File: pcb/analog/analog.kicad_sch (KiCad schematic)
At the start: 65 parts, among them J1 USB_C_Receptacle_USB2.0, SW1 SW_Push, SW2 SW_Push, U1 SRV05-4, U2 XC6206P332MR, U3 DRV5056A3xDBZxQ1, U4 DRV5056A3xDBZxQ1, U5 DRV5056A3xDBZxQ1, U6 74AHCT1G125, U7 74AHCT1G125, U8 RP2040, U9 W25Q128JVS, Y1 12MHz

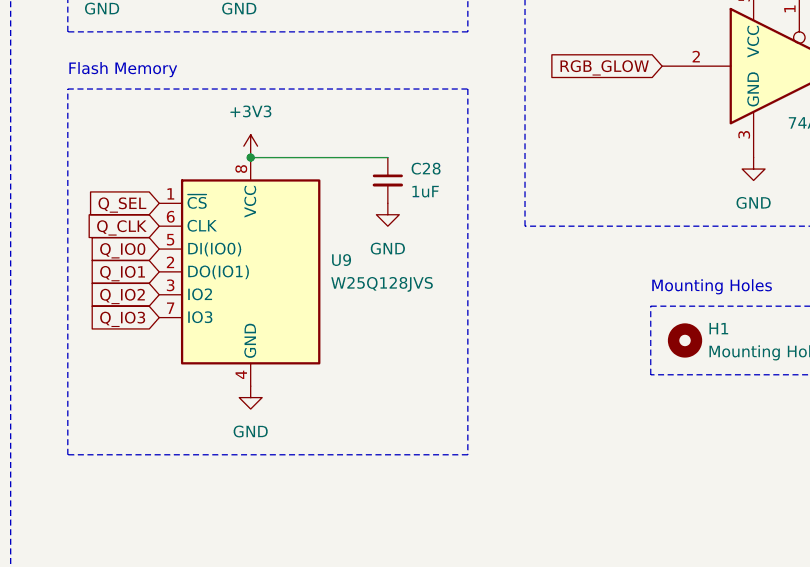
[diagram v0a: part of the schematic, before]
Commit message: feat: setup bom and initial gerbers files
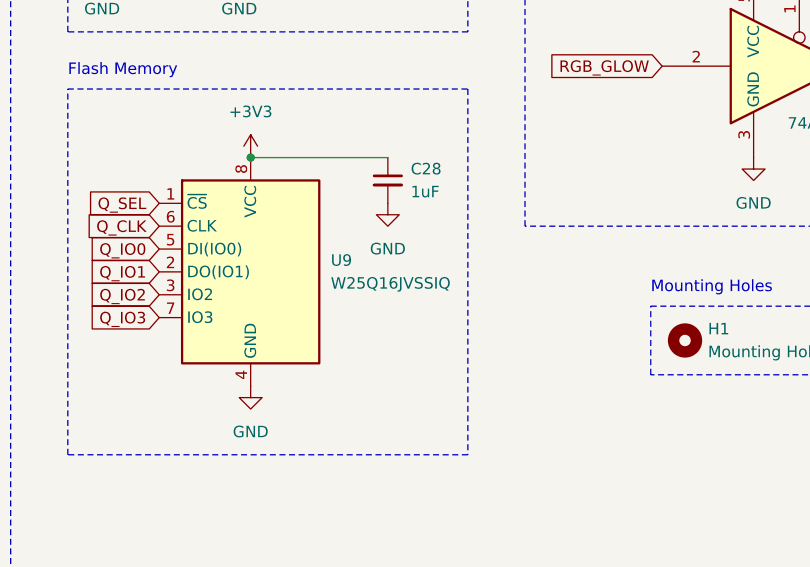
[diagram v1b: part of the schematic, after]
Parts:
- C1, C12, C16, C2, C28, C3, C4, C5, C6, C7, C8: LCSC (none) -> C52923
- C10, C11, C13, C14, C17, C18, C19, C20, C21, C22, C23, C26, C27, C9: LCSC (none) -> C1525
- C15: LCSC (none) -> C19702
- C24, C25: LCSC (none) -> C1555
- D1, D2: LCSC (none) -> C2761795
- F1: LCSC (none) -> C170165
- J1: LCSC (none) -> C165948
- LED1, LED2, LED3: LCSC (none) -> C5149201
- R1, R10, R12, R13, R2: LCSC (none) -> C25905
- R11, R9: LCSC (none) -> C25100
- R14, R6, R7, R8: LCSC (none) -> C11702
- R3, R4, R5: LCSC (none) -> C25076
- SW1, SW2: LCSC (none) -> C318884
- U1: LCSC (none) -> C2836319
- U2: LCSC (none) -> C5446
- U3, U4, U5: LCSC (none) -> C2152965
- U6, U7: LCSC (none) -> C151417
- U8: LCSC (none) -> C2040
- U9: value W25Q128JVS -> W25Q16JVSSIQ; LCSC (none) -> C131025
- Y1: LCSC (none) -> C9002
